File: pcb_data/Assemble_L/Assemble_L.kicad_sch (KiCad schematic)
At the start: 75 parts, among them U1 XIAO-nRF52840-DIP

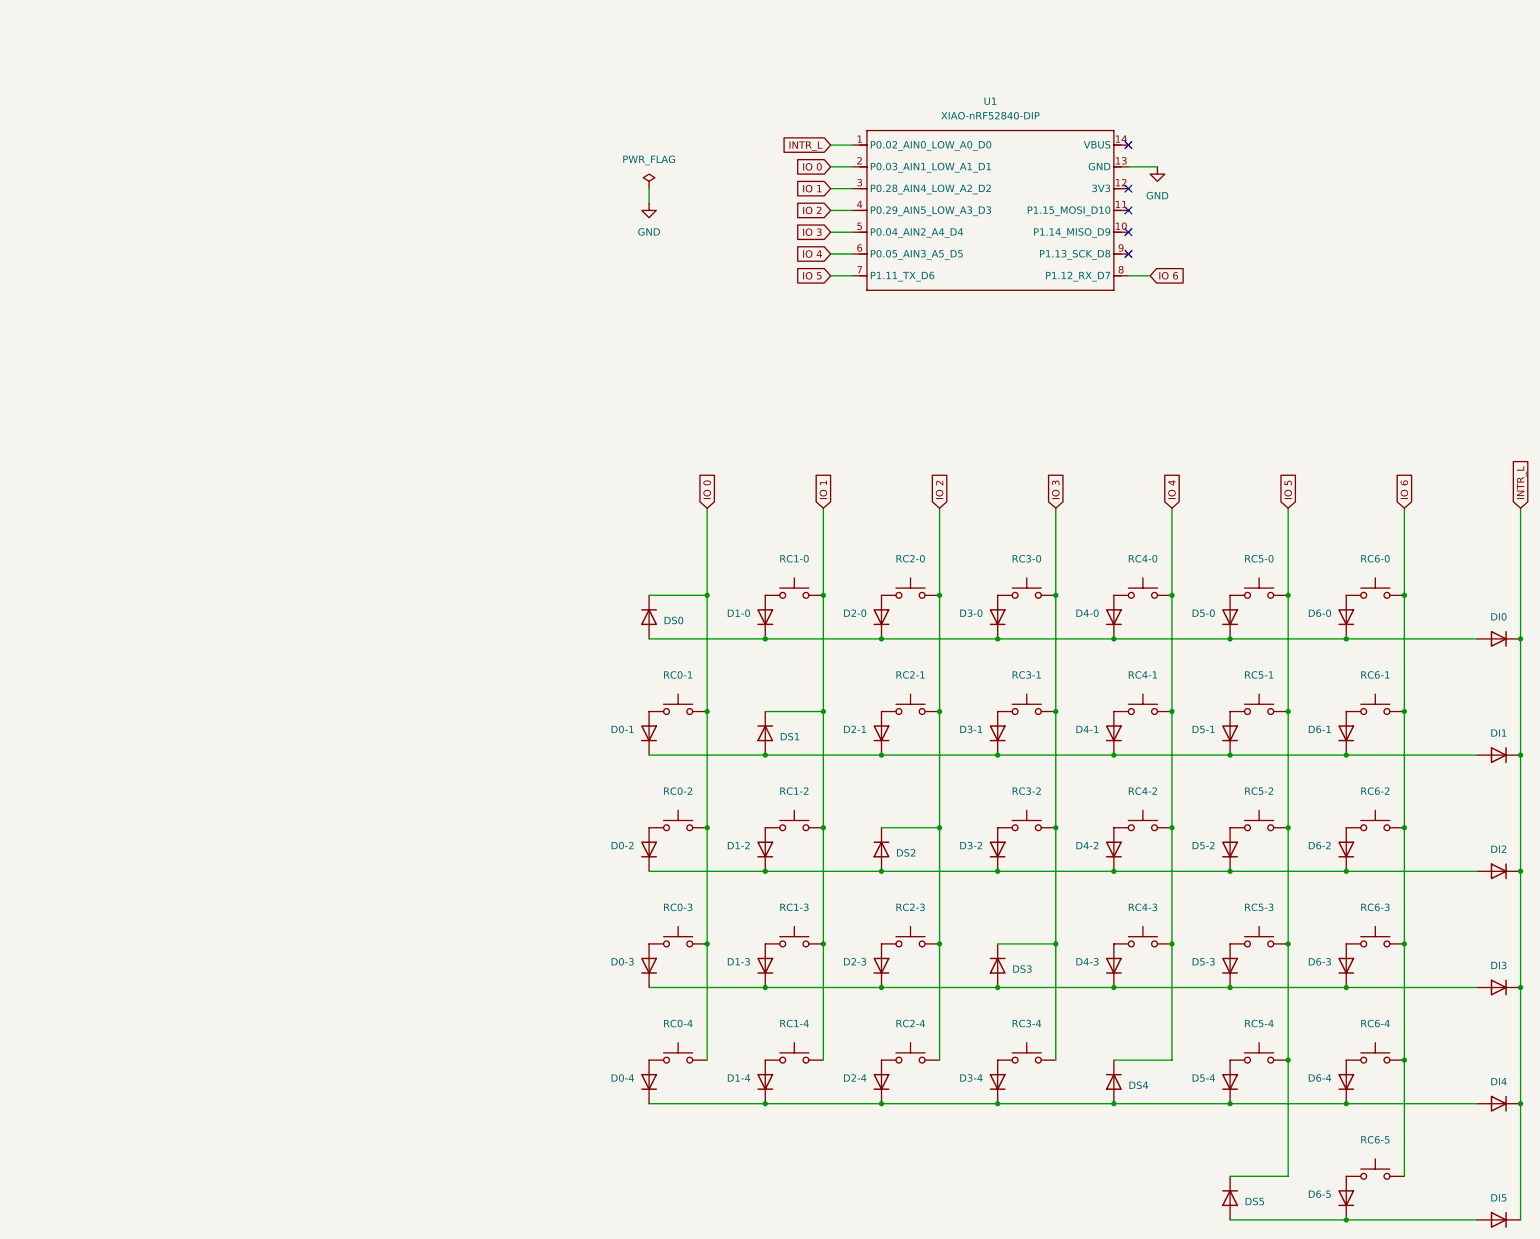
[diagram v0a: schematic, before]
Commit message: update symbol
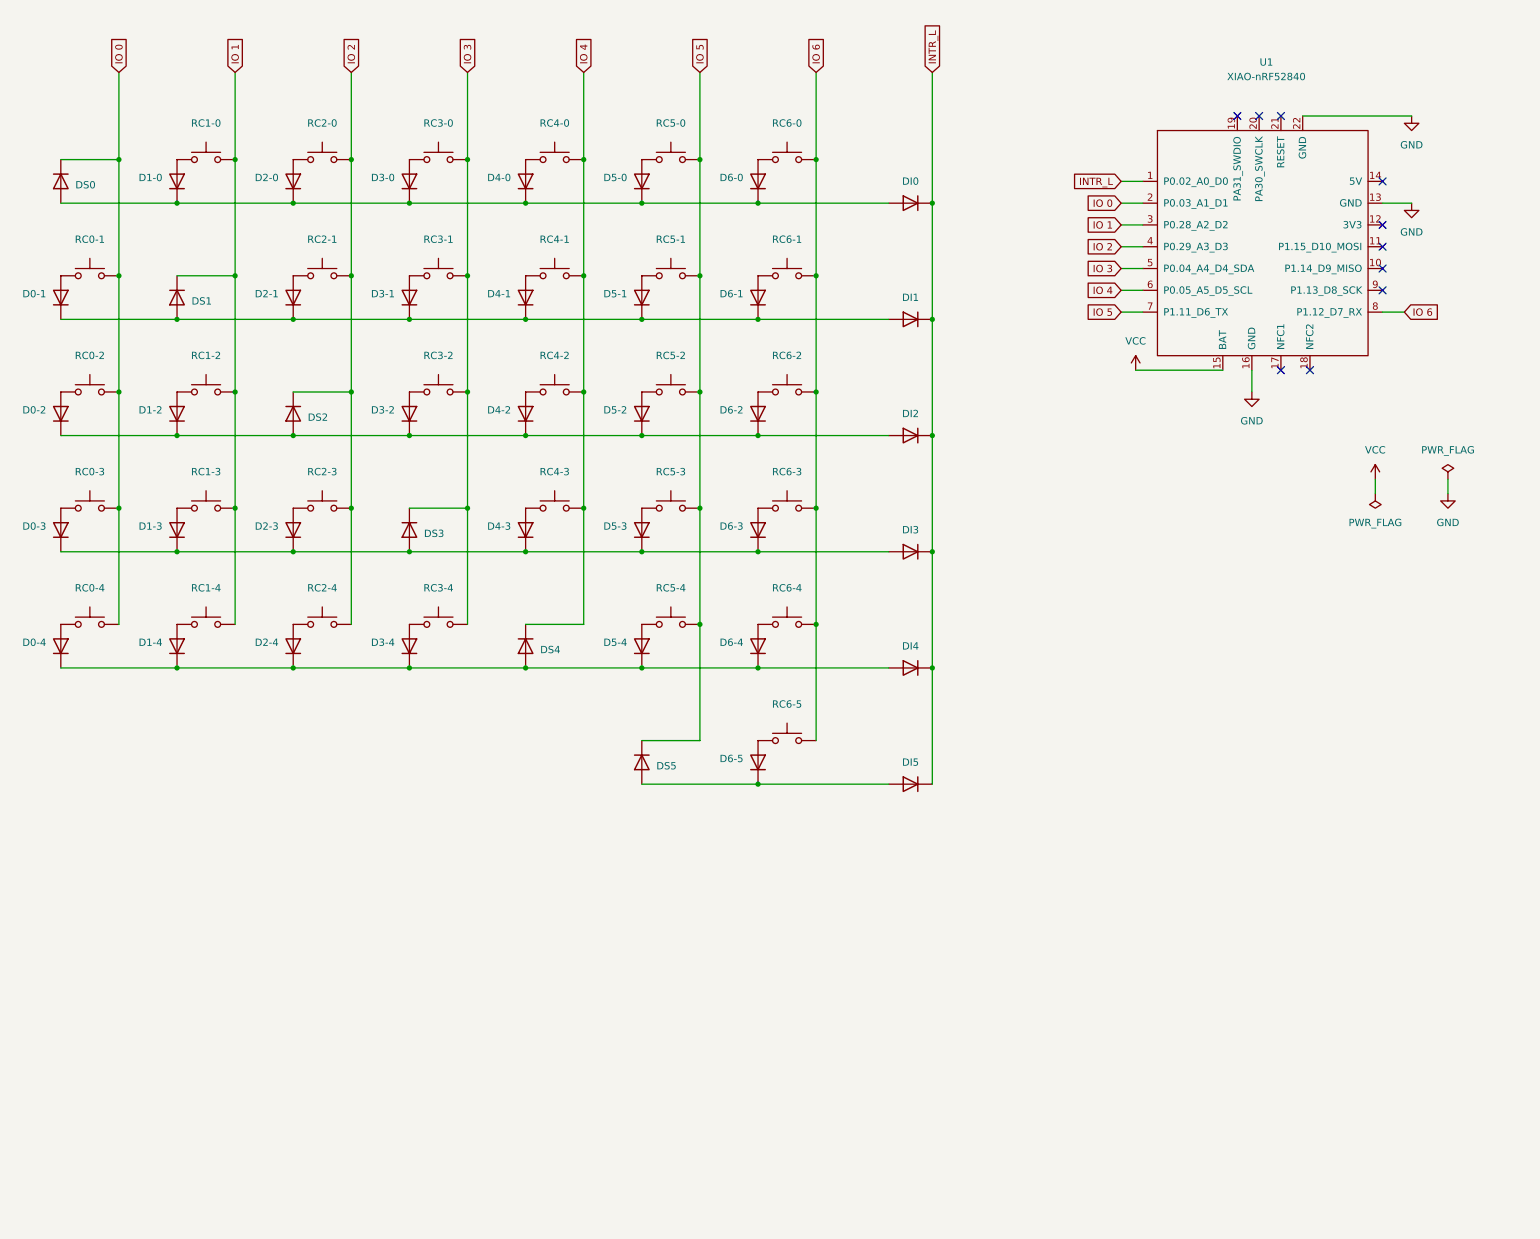
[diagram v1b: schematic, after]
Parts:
- U1: value XIAO-nRF52840-DIP -> XIAO-nRF52840; footprint Seeed Studio XIAO Series Library:XIAO-nRF52840-DIP -> custom-library:XIAO-nRF52840; symbol Seeed_Studio_XIAO_Series:XIAO-nRF52840-DIP -> Seeed_Studio_XIAO_Series:XIAO-nRF52840-SMD
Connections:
- net GND: now also U1.16 (GND), U1.22 (GND)
- new net VCC: U1.15 (BAT)
- no-connect marks 5 -> 10
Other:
- moved on the sheet: D0-1, D0-2, D0-3, D0-4, D1-0, D1-2, D1-3, D1-4, D2-0, D2-1, D2-3, D2-4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
